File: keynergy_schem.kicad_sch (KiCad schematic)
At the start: 11 parts, among them J1 Conn_01x05_Pin, J2 Conn_01x02_Pin, SW1 SW_DPDT_x2, SW2 SW_DPDT_x2, SW3 SW_DPDT_x2, SW4 SW_DPDT_x2

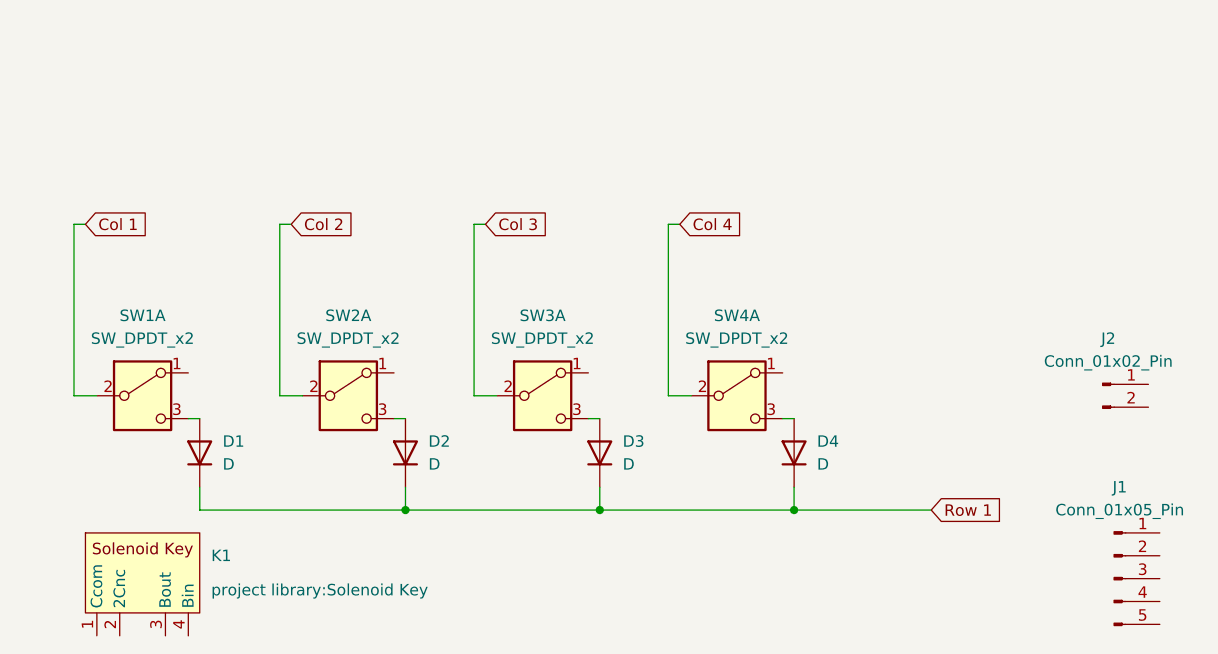
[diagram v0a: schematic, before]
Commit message: new files
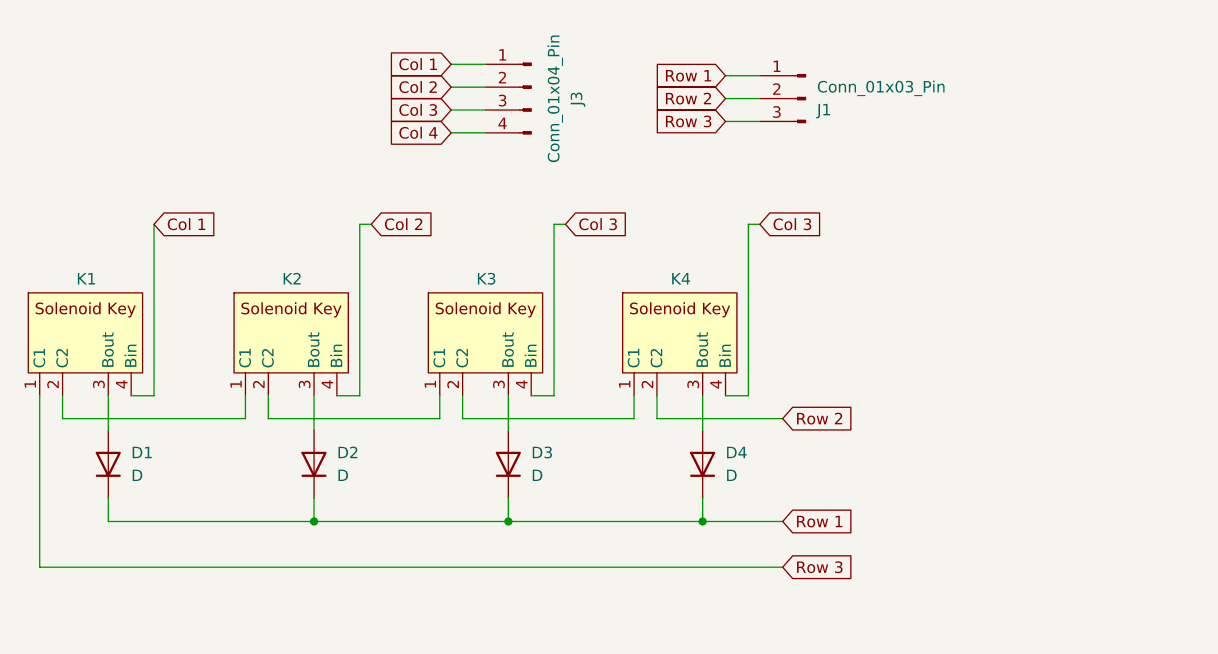
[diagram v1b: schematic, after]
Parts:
- removed J1: Conn_01x05_Pin, symbol Connector:Conn_01x05_Pin
- removed J2: Conn_01x02_Pin, symbol Connector:Conn_01x02_Pin
- removed SW1, SW2, SW3, SW4: SW_DPDT_x2, symbol Switch:SW_DPDT_x2
- added J1: Conn_01x03_Pin, Connector_PinHeader_2.54mm:PinHeader_1x03_P2.54mm_Vertical, symbol Connector:Conn_01x03_Pin
- added J3: Conn_01x04_Pin, Connector_PinHeader_2.54mm:PinHeader_1x04_P2.54mm_Vertical, symbol Connector:Conn_01x04_Pin
- added K2, K3, K4: ~, project library:Solenoid Key, symbol Key_symbol:Solenoid_Key
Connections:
- net Col 1: now also K1.4 (Bin), J3.1 (Pin_1)
- net Col 2: now also J3.2 (Pin_2), K2.4 (Bin)
- net Col 3: now also J3.3 (Pin_3), K3.4 (Bin), K4.4 (Bin)
- net Col 4: now also J3.4 (Pin_4)
- net Row 1: now also J1.1 (Pin_1)
- net at D1.2 (A): now also K1.3 (Bout)
- net at D3.2 (A): now also K3.3 (Bout)
- net at D2.2 (A): now also K2.3 (Bout)
- net Row 3: now reaches K1.1 (C1)
- net Row 3: now also J1.3 (Pin_3)
- net at K1.2 (C2): now also K2.1 (C1)
- net at D4.2 (A): now also K4.3 (Bout)
- new net: K2.2 (C2), K3.1 (C1)
- new net: K3.2 (C2), K4.1 (C1)
- new net Row 2: J1.2 (Pin_2), K4.2 (C2)
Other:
- moved on the sheet: D1, D2, D3, D4, K1
